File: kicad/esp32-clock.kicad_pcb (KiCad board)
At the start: 2 copper layers, 33 parts, among them J1 Battery Connector, P1 USB_C_Plug_USB2.0, SW1 RESET, SW2 BOOT, U1 ESP-12E, U2 CP2102N-Axx-xQFN20, U3 MCP73831-2-OT, U4 BCM857BS, U5 ME6211H33M5G

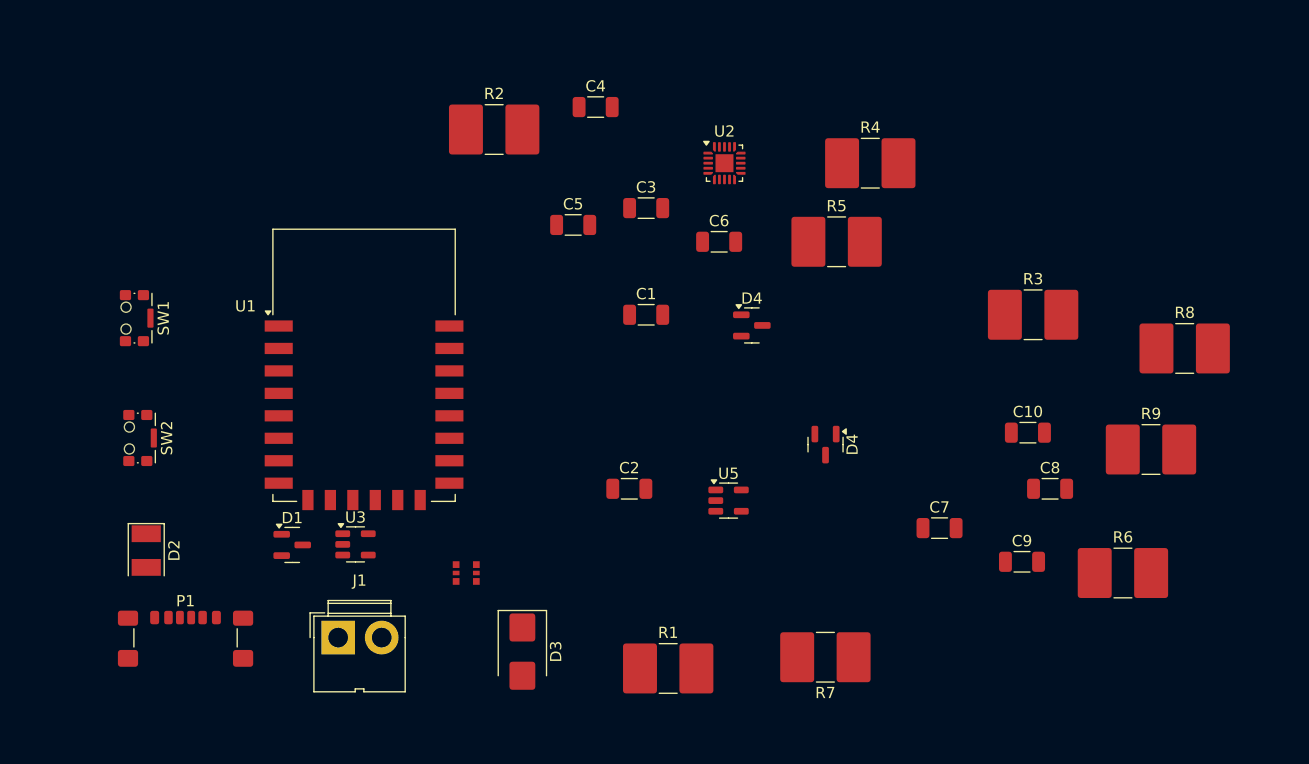
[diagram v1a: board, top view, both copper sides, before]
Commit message: init
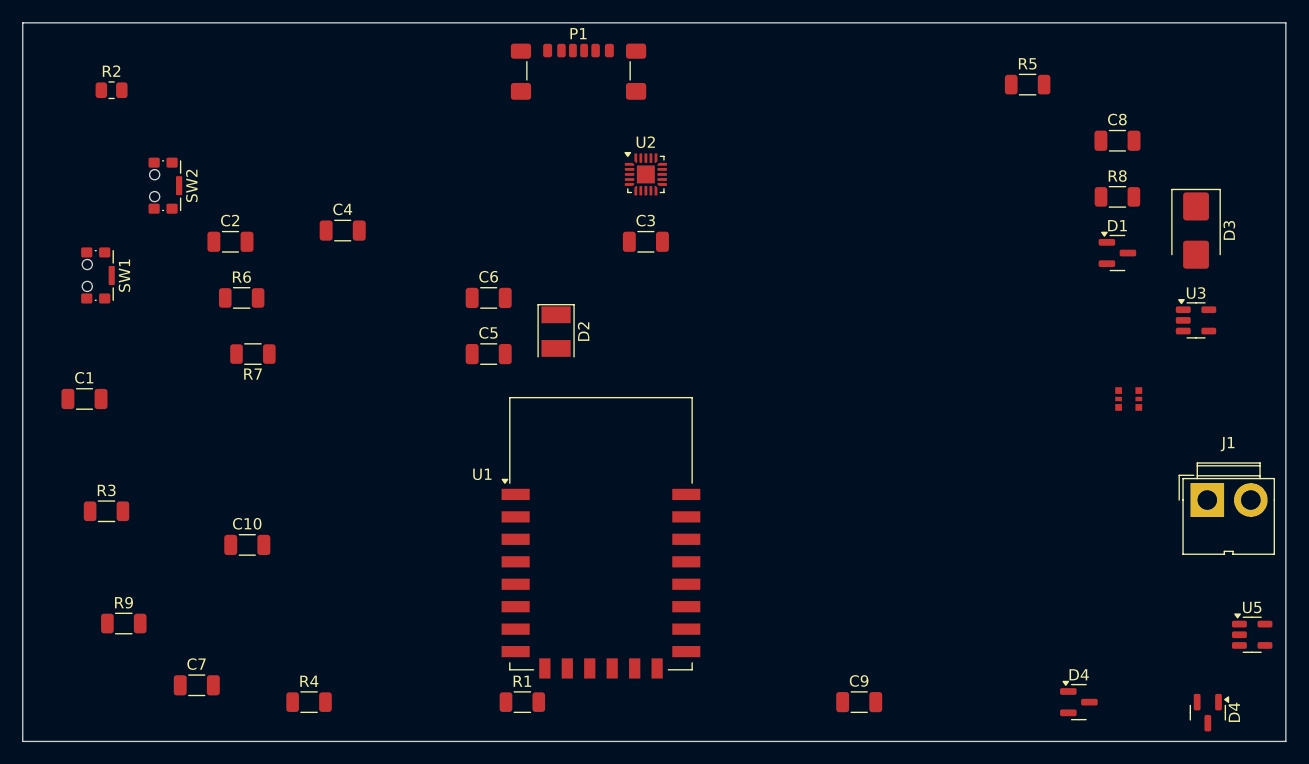
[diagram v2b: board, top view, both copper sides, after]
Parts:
- R1, R3, R4, R5, R6, R7, R8, R9: footprint Resistor_SMD:R_2816_7142Metric -> Resistor_SMD:R_1206_3216Metric
- R2: footprint Resistor_SMD:R_2816_7142Metric -> Resistor_SMD:R_0805_2012Metric
- moved R9 92.8 mm to (70.5, 104.0)
- moved R3 84.4 mm to (69.0, 94.0)
- moved R6 82.2 mm to (81.0, 75.0)
- moved J1 78.4 mm to (167.0, 93.0)
- moved D1 78.0 mm to (159.0, 71.0)
- moved U3 77.5 mm to (166.0, 77.0)
- moved D3 70.8 mm to (166.0, 69.0)
- moved C10 70.2 mm to (81.5, 97.0)
- moved R4 69.3 mm to (87.0, 111.0)
- moved C7 67.6 mm to (77.0, 109.5)
- moved P1 61.4 mm to (111.0, 56.0)
- moved U4 61.0 mm to (160.0, 84.0)
- moved R7 57.7 mm to (82.0, 80.0)
- moved C1 50.6 mm to (67.0, 84.0)
- moved U5 48.1 mm to (171.0, 105.0)
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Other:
- board outline added: 112.5 x 64 mm
